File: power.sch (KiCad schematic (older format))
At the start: 23 parts

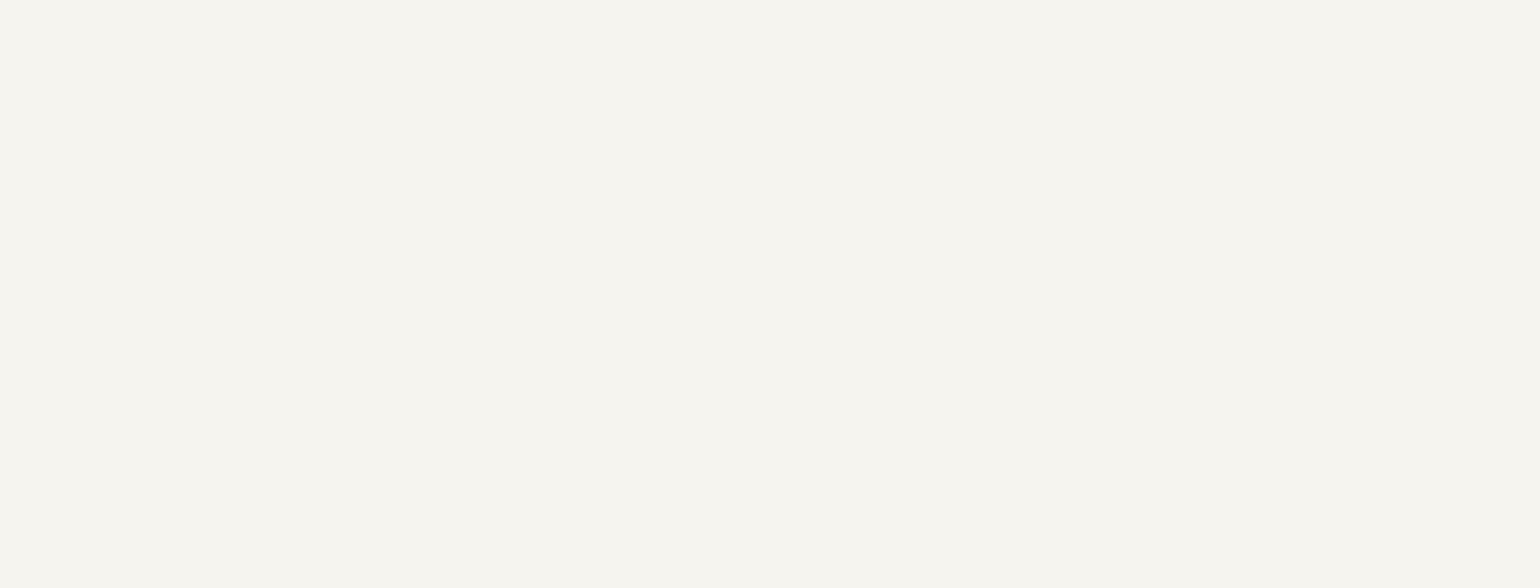
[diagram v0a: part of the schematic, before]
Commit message: update,
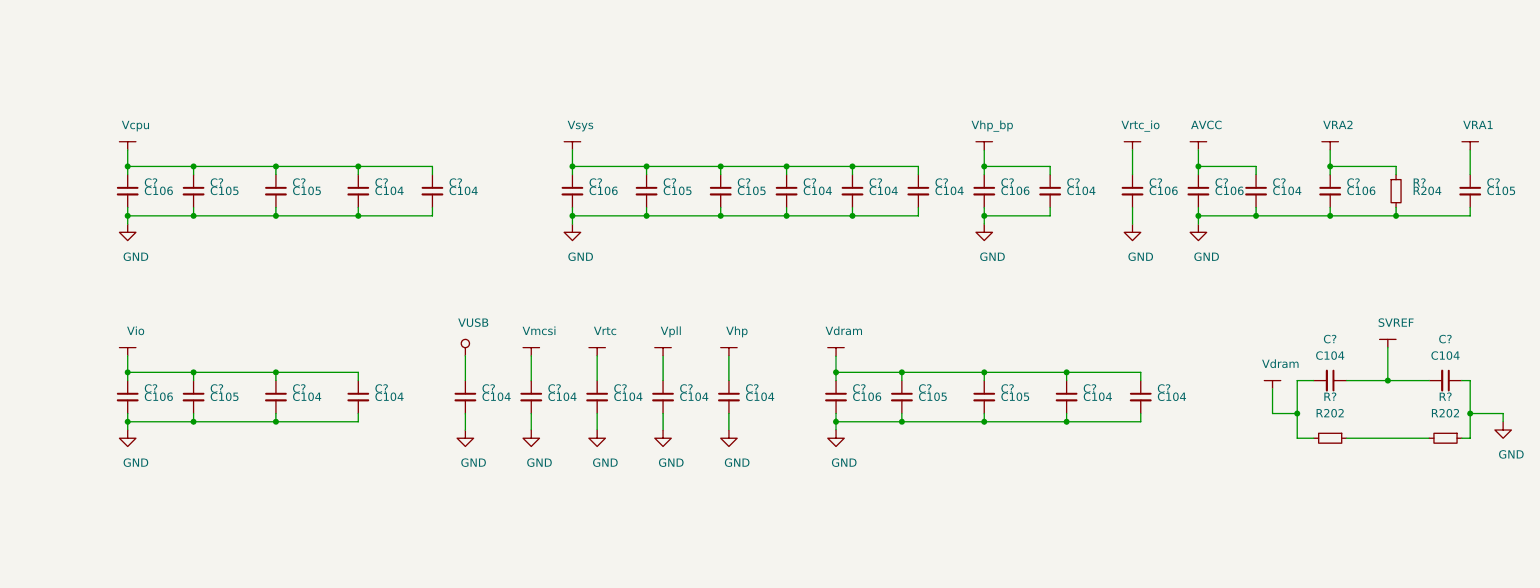
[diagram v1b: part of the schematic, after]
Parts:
- added C? (x8): C106, symbol taobao-c:C106
- added C? (x8): C105, symbol taobao-c:C105
- added C? (x6): C104, symbol taobao-c:C105
- added C? (x12): C104, symbol taobao-c:C104
- added R?: R204, symbol taobao-r:R204
- added R? (x2): R202, symbol taobao-r:R202
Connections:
- net +1V2: now also C?.1, C?.1, C?.1, C?.1, C?.1, C?.1, C?.1, C?.1, C?.1, C?.1, C?.1
- net +1V8: now also C?.1, C?.1, C?.1, C?.1, C?.1, C?.2, R?.2
- net +3V0: now also C?.1, C?.1, C?.1
- net +3V3: now also C?.1, C?.1, C?.1, C?.1, C?.1, C?.1, C?.1
- net GND: now also C?.1, C?.2, C?.2, C?.2, C?.2, C?.2, C?.2, C?.2, C?.2, C?.2, C?.2, C?.2, C?.2, C?.2, C?.2, C?.2, C?.2, C?.2, C?.2, C?.2, C?.2, C?.2, C?.2, C?.2, C?.2, C?.2, C?.2, C?.2, C?.2, C?.2, C?.2, C?.2, C?.2, R?.1, R?.2
- net Vrtc: now also C?.1
- new net: R?.1, R?.2
- new net SVREF: C?.1, C?.2
- new net VRA1: C?.1
- new net VRA2: C?.1, R?.1
- new net Vhp_bp: C?.1, C?.1
- new net Vrtc_io: C?.1
